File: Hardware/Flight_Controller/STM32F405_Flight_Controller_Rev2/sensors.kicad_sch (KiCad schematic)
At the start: 7 parts, among them U2 ICM-42688-P, U3 BMP390L

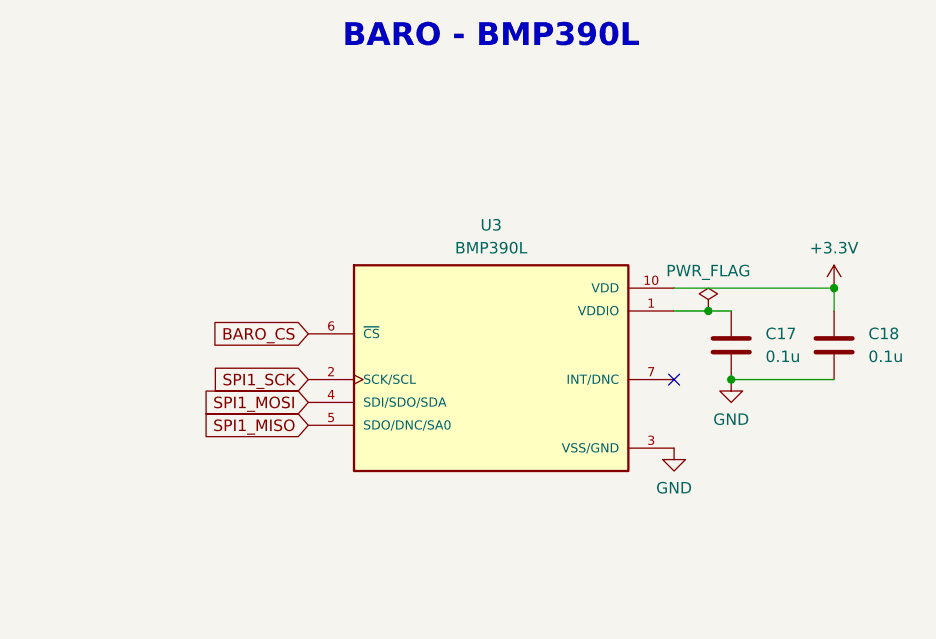
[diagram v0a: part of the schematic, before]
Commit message: Ready Rev2 PCB
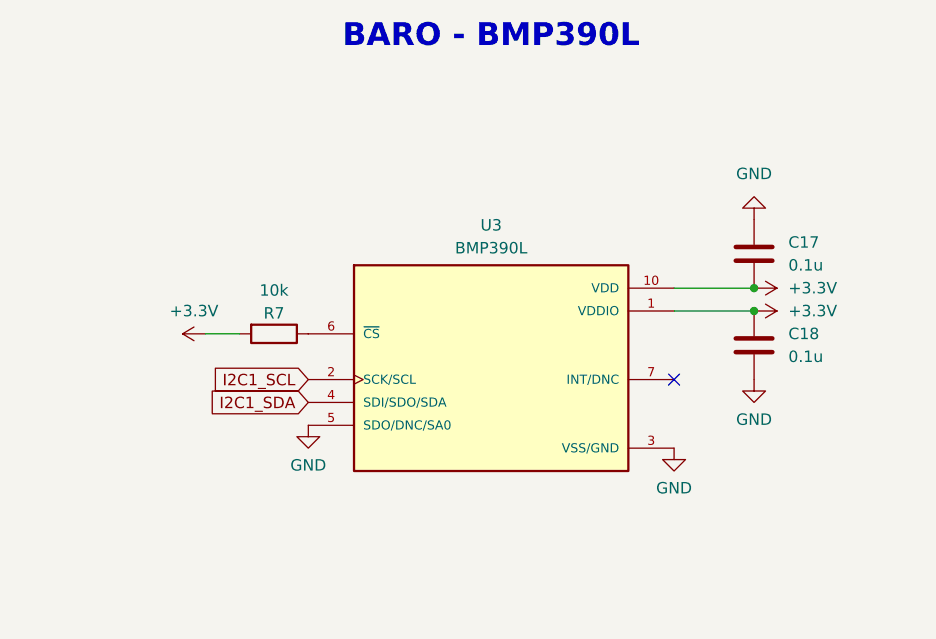
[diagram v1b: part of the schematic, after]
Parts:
- added R7: 10k, Resistor_SMD:R_0603_1608Metric_Pad0.98x0.95mm_HandSolder, symbol Device:R
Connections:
- net +3.3V: now also C17.1, U3.1 (VDDIO), R7.2
- net GND: now also U3.5 (SDO/DNC/SA0)
- net SPI1_MISO: no longer U3.5 (SDO/DNC/SA0)
- net SPI1_MOSI: no longer U3.4 (SDI/SDO/SDA)
- net SPI1_SCK: no longer U3.2 (SCK/SCL)
- net BARO_CS: no longer names the net of U3.6 (~{CS})
- net BARO_CS: now also R7.1
- new net I2C1_SCL: U3.2 (SCK/SCL)
- new net I2C1_SDA: U3.4 (SDI/SDO/SDA)
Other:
- moved on the sheet: C17, C18
